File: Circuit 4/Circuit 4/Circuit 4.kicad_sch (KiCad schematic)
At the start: 49 parts, among them SW1 SW_DIP_x01, SW2 SW_DIP_x08, SW3 Submit, SW4 Reset, U1 7404, U10 74LS283, U11 74LS74, U12 74LS74, U13 74LS74, U14 74LS74, U15 74LS74, U16 74LS74, U17 74LS74, U18 74LS74, U2 7408, U3 7404, U4 7408, U5 74LS86, U6 74LS86, U7 74HC86, U8 7432, U9 74LS283

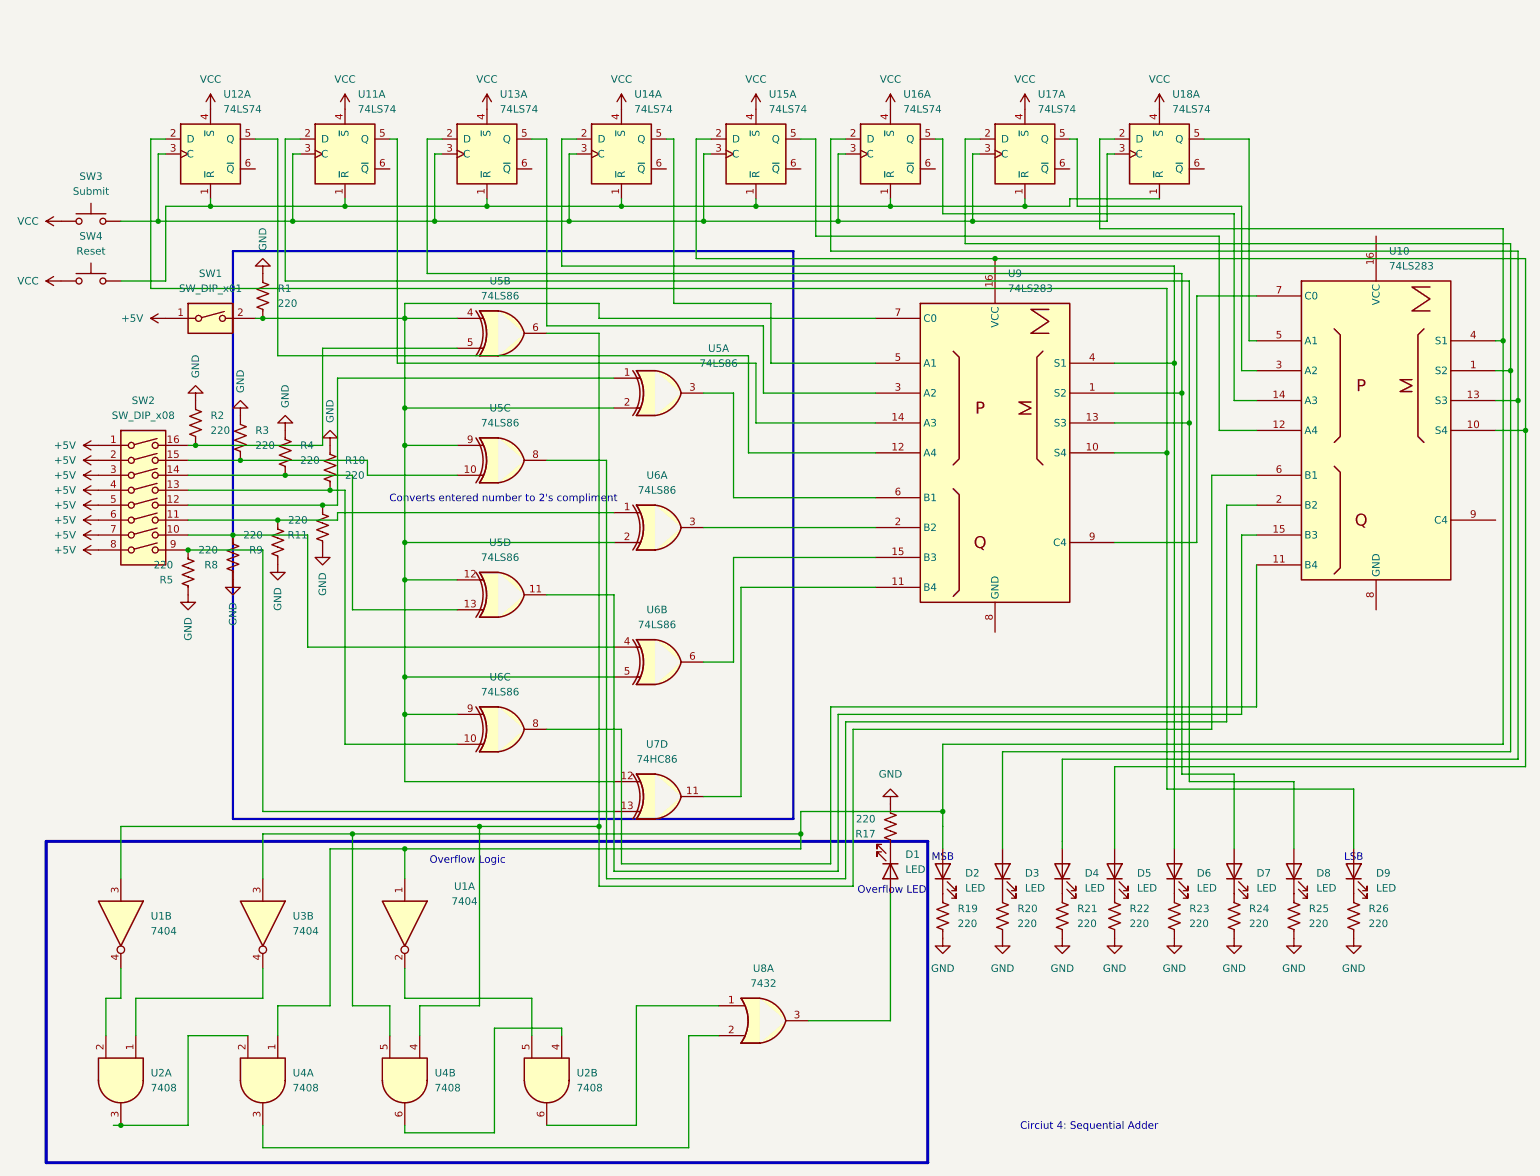
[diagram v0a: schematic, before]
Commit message: Add files via upload
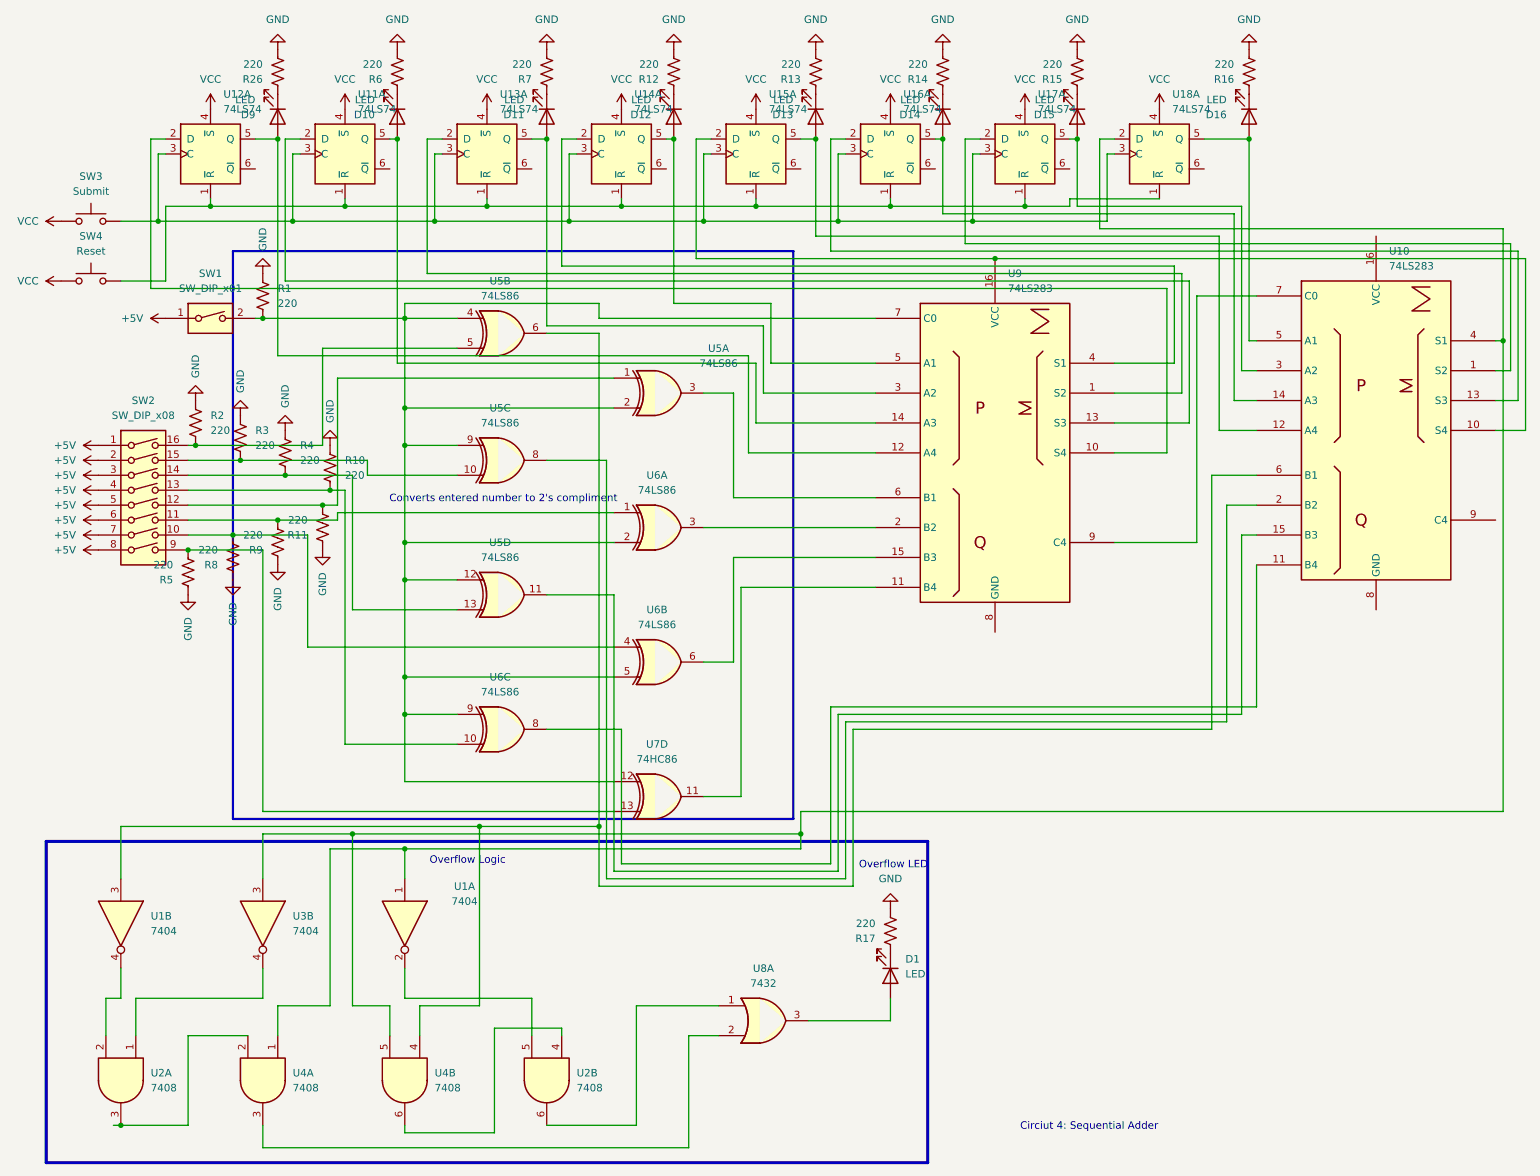
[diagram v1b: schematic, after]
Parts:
- removed D2, D3, D4, D5, D6, D7, D8: LED, symbol Device:LED
- removed R19, R20, R21, R22, R23, R24, R25: 220, symbol Device:R_US
- added D10, D11, D12, D13, D14, D15, D16: LED, symbol Device:LED
- added R12, R13, R14, R15, R16, R6, R7: 220, symbol Device:R_US
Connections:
- net GND: now also R12.2, R13.2, R14.2, R15.2, R16.2, R6.2, R7.2
- net at U12.2 (D), U9.10 (S4): no longer D9.2 (A)
- net at U12.5 (Q), U9.12 (A4): now also D9.2 (A)
- net at U11.5 (Q), U9.14 (A3): now also D10.2 (A)
- net at U13.5 (Q), U9.3 (A2): now also D11.2 (A)
- net at U14.5 (Q), U9.5 (A1): now also D12.2 (A)
- net at U10.12 (A4), U15.5 (Q): now also D13.2 (A)
- net at U10.14 (A3), U16.5 (Q): now also D14.2 (A)
- net at U10.3 (A2), U17.5 (Q): now also D15.2 (A)
- net at U10.5 (A1), U18.5 (Q): now also D16.2 (A)
- new net: D14.1 (K), R14.1
- new net: D13.1 (K), R13.1
- new net: D16.1 (K), R16.1
- new net: D11.1 (K), R7.1
- new net: D12.1 (K), R12.1
- new net: D15.1 (K), R15.1
- new net: D10.1 (K), R6.1
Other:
- note removed: "LSB"
- note removed: "MSB"
- moved on the sheet: D1, D9, R17, R26
